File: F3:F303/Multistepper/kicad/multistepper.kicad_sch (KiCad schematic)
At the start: 14 parts, among them J8 USB_B, J9 Screw_Terminal_01x03, Q1 B0505S, SW3 SW_DIP_x01, U2 ISO1050DUB, U3 USBLC6-2SC6

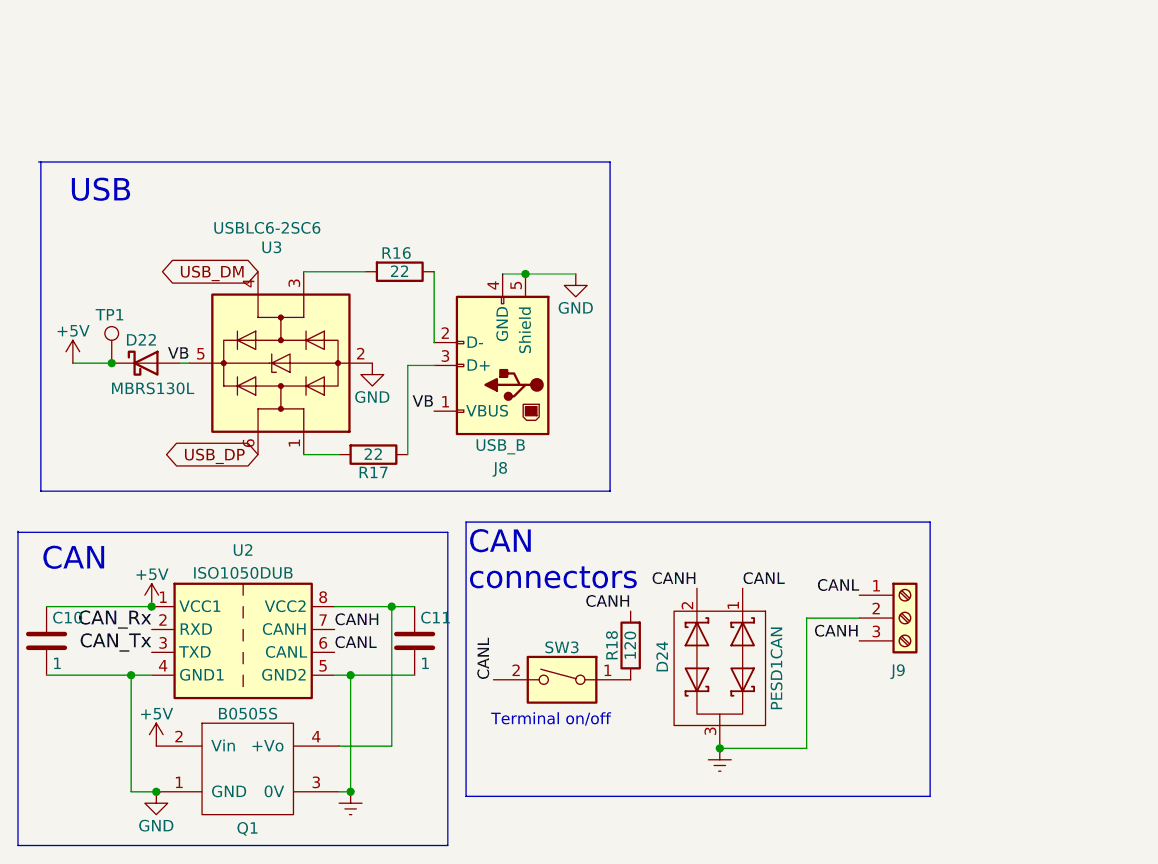
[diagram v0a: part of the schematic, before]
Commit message: multistepper: cont
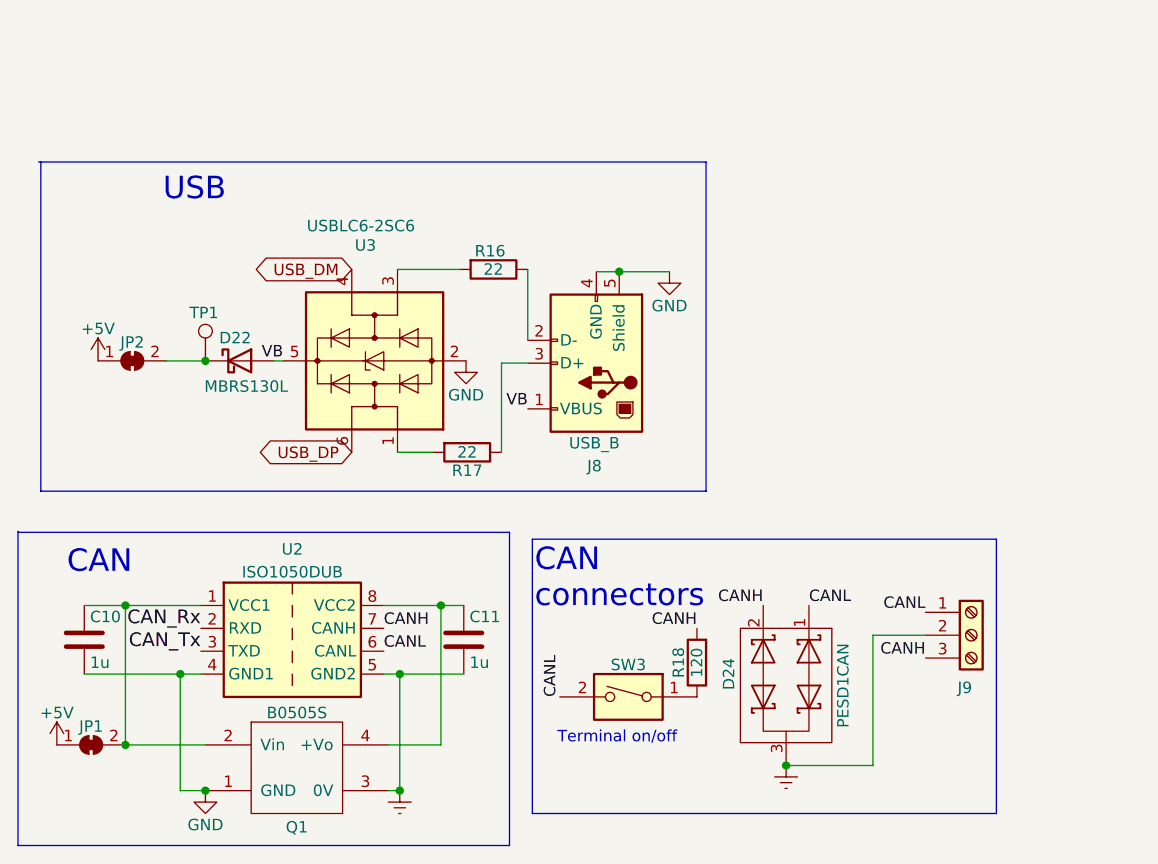
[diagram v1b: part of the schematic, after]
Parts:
- added JP1, JP2: SolderJumper_2_Bridged, Jumper:SolderJumper-2_P1.3mm_Open_TrianglePad1.0x1.5mm, symbol Jumper:SolderJumper_2_Bridged
- C10, C11: value 1 -> 1u; footprint Capacitor_SMD:C_0805_2012Metric_Pad1.15x1.40mm_HandSolder -> Capacitor_SMD:C_0603_1608Metric_Pad1.08x0.95mm_HandSolder
- Q1: footprint my_footprints:B0x0xS -> stepper:B0x0xS
- R16, R17: footprint Resistor_SMD:R_0603_1608Metric_Pad1.05x0.95mm_HandSolder -> Resistor_SMD:R_0603_1608Metric_Pad0.98x0.95mm_HandSolder
- R18: footprint Resistor_SMD:R_1210_3225Metric_Pad1.42x2.65mm_HandSolder -> Resistor_SMD:R_1210_3225Metric_Pad1.30x2.65mm_HandSolder
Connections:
- net +5V: now also JP1.1 (A), JP2.1 (A); no longer C10.1, D22.1 (K), Q1.2 (Vin), TP1.1, U2.1 (VCC1)
- new net: D22.1 (K), JP2.2 (B), TP1.1
- new net: C10.1, JP1.2 (B), Q1.2 (Vin), U2.1 (VCC1)
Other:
- moved on the sheet: C10, C11, D22, D24, J8, J9, Q1, R16, R17, R18, SW3, TP1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

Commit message: multistepper schematic
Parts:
- TP1: value 5V -> 5Vusb
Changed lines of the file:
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@@
       (effects (font (size 1.27 1.27)) (justify left))
     )
-    (property "Value" "5V" (id 1) (at 37.7952 139.7762 0)
+    (property "Value" "5Vusb" (id 1) (at 37.7952 139.7762 0)
       (effects (font (size 1.27 1.27)) (justify left) hide)
     )
@@
       (reference "#PWR03") (unit 1) (value "GND") (footprint "")
     )
-    (path "/076c38b6-e164-46bb-9d96-26f8bdfeca37/99206ade-04b2-46fa-85f1-261359dfd31b"
-      (reference "#PWR04") (unit 1) (value "+3V3") (footprint "")
-    )
     (path "/076c38b6-e164-46bb-9d96-26f8bdfeca37/f5301934-7edc-46db-ae48-58199dc2aa43"
       (reference "#PWR05") (unit 1) (value "GND") (footprint "")
@@
       (reference "#PWR08") (unit 1) (value "+3V3") (footprint "")
     )
-    (path "/076c38b6-e164-46bb-9d96-26f8bdfeca37/2b033d26-211f-47c5-ad30-9cb9aea659a6"
-      (reference "#PWR09") (unit 1) (value "+3V3") (footprint "")
-    )
-    (path "/076c38b6-e164-46bb-9d96-26f8bdfeca37/73b1df7f-a887-48b4-9ce7-3d8db7403e95"
-      (reference "#PWR010") (unit 1) (value "+3V3") (footprint "")
-    )
     (path "/076c38b6-e164-46bb-9d96-26f8bdfeca37/4d6a594b-d668-48f8-8d40-146959ef7aa5"
       (reference "#PWR011") (unit 1) (value "GND") (footprint "")
@@
       (reference "#PWR041") (unit 1) (value "GND") (footprint "")
     )
-    (path "/cf2c4fa9-a57e-4812-ae0c-3db57f6071a5/610893b8-7125-40df-867c-22854f8efd58/4f508297-4488-4315-85eb-5261f9d02134"
-      (reference "#PWR042") (unit 1) (value "+3.3V") (footprint "")
+    (path "/076c38b6-e164-46bb-9d96-26f8bdfeca37/4354a899-4f12-4b14-9a0f-0357b172479a"
+      (reference "#PWR042") (unit 1) (value "GND") (footprint "")
     )
     (path "/076c38b6-e164-46bb-9d96-26f8bdfeca37/c9d2b617-3560-41ef-a3a7-a6d08311dfc5"
@@
       (reference "#PWR0124") (unit 1) (value "GND") (footprint "")
     )
-    (path "/076c38b6-e164-46bb-9d96-26f8bdfeca37/b26d12d8-b821-4fbb-bcf0-02f1fc523839"
-      (reference "#PWR0125") (unit 1) (value "+3V3") (footprint "")
-    )
     (path "/076c38b6-e164-46bb-9d96-26f8bdfeca37/b728d2bc-216a-439f-be0d-9040aecbd583"
       (reference "C1") (unit 1) (value "12") (footprint "Capacitor_SMD:C_0603_1608Metric_Pad1.08x0.95mm_HandSolder")
@@
     )
     (path "/076c38b6-e164-46bb-9d96-26f8bdfeca37/9eb0e3e4-2412-4862-9254-ebfae0e788ab"
-      (reference "J2") (unit 1) (value "buttons_I2C") (footprint "Connector_IDC:IDC-Header_2x05_P2.54mm_Vertical")
+      (reference "J2") (unit 1) (value "Buttons/I2C") (footprint "Connector_IDC:IDC-Header_2x05_P2.54mm_Vertical")
     )
     (path "/076c38b6-e164-46bb-9d96-26f8bdfeca37/3b30193d-b3cb-42a8-a75c-e3cbeadeeead"
-      (reference "J3") (unit 1) (value "screen") (footprint "Connector_IDC:IDC-Header_2x05_P2.54mm_Vertical")
+      (reference "J3") (unit 1) (value "Screen") (footprint "Connector_IDC:IDC-Header_2x05_P2.54mm_Vertical")
     )
     (path "/beac4271-940a-4bcd-9fa5-ece775a07d41/ad1d252e-a412-4fd5-af6f-3bf5db8aac83"
@@
     )
     (path "/076c38b6-e164-46bb-9d96-26f8bdfeca37/23242767-ce55-4623-97c5-9de9c42c2a3f"
-      (reference "J7") (unit 1) (value "ADC2") (footprint "Connector_JST:JST_PH_B4B-PH-K_1x04_P2.00mm_Vertical")
+      (reference "J7") (unit 1) (value "GPO") (footprint "Connector_JST:JST_PH_B4B-PH-K_1x04_P2.00mm_Vertical")
     )
     (path "/0fd87c97-8042-4653-abdd-7019b1430685"
@@
       (reference "J10") (unit 1) (value "Screw_Terminal_01x02") (footprint "TerminalBlock_Phoenix:TerminalBlock_Phoenix_MKDS-1,5-2_1x02_P5.00mm_Horizontal")
     )
-    (path "/cf2c4fa9-a57e-4812-ae0c-3db57f6071a5/610893b8-7125-40df-867c-22854f8efd58/0f165469-1249-4064-aadf-0fc6a85a60f4"
-      (reference "J11") (unit 1) (value "Conn_01x03_Male") (footprint "Connector_PinHeader_2.54mm:PinHeader_1x03_P2.54mm_Vertical")
-    )
     (path "/cf2c4fa9-a57e-4812-ae0c-3db57f6071a5/610893b8-7125-40df-867c-22854f8efd58/0f3f2180-6e00-4de5-8d6d-bb200c241b76"
-      (reference "J12") (unit 1) (value "Conn_01x03_Male") (footprint "Connector_PinHeader_2.54mm:PinHeader_1x03_P2.54mm_Vertical")
+      (reference "J11") (unit 1) (value "LimS") (footprint "Connector_JST:JST_EH_B4B-EH-A_1x04_P2.50mm_Vertical")
     )
     (path "/cf2c4fa9-a57e-4812-ae0c-3db57f6071a5/610893b8-7125-40df-867c-22854f8efd58/e602956b-fb1a-48e1-af9c-9935214ce0ab"
-      (reference "J13") (unit 1) (value "Conn_01x04_Male") (footprint "Connector_PinHeader_2.54mm:PinHeader_1x04_P2.54mm_Vertical")
+      (reference "J12") (unit 1) (value "Stepper") (footprint "Connector_JST:JST_EH_B4B-EH-A_1x04_P2.50mm_Vertical")
+    )
+    (path "/076c38b6-e164-46bb-9d96-26f8bdfeca37/8a056ff3-5fc5-445e-813f-5479481ae2be"
+      (reference "J13") (unit 1) (value "UART") (footprint "Connector_JST:JST_PH_B3B-PH-K_1x03_P2.00mm_Vertical")
     )
     (path "/e07df136-9c14-457d-8c74-2e7051ea67ac"
@@
       (reference "JP15") (unit 1) (value "SolderJumper_2_Bridged") (footprint "Jumper:SolderJumper-2_P1.3mm_Open_TrianglePad1.0x1.5mm")
     )
-    (path "/cf2c4fa9-a57e-4812-ae0c-3db57f6071a5/610893b8-7125-40df-867c-22854f8efd58/19b709bd-064d-431e-981a-21d8140226f7"
-      (reference "JP16") (unit 1) (value "SolderJumper_2_Bridged") (footprint "Jumper:SolderJumper-2_P1.3mm_Open_TrianglePad1.0x1.5mm")
-    )
-    (path "/cf2c4fa9-a57e-4812-ae0c-3db57f6071a5/610893b8-7125-40df-867c-22854f8efd58/9a737b0c-0674-4408-94a4-2d0cb4f1ebe2"
-      (reference "JP17") (unit 1) (value "SolderJumper_2_Bridged") (footprint "Jumper:SolderJumper-2_P1.3mm_Open_TrianglePad1.0x1.5mm")
-    )
     (path "/916f71ef-9b2f-424f-a64d-0b6af99b627f/b3fc53d8-12ed-4d5b-adca-e33d10eb8430"
       (reference "L1") (unit 1) (value "100u") (footprint "Inductor_THT:L_Toroid_Horizontal_D6.5mm_P10.00mm_Diameter7-5mm_Amidon-T25")
@@
       (reference "R23") (unit 1) (value "100") (footprint "Resistor_SMD:R_0603_1608Metric_Pad0.98x0.95mm_HandSolder")
     )
+    (path "/076c38b6-e164-46bb-9d96-26f8bdfeca37/d42c91a2-1307-4ab7-930f-7f9359c5d693"
+      (reference "R24") (unit 1) (value "22") (footprint "Resistor_SMD:R_0603_1608Metric_Pad0.98x0.95mm_HandSolder")
+    )
+    (path "/076c38b6-e164-46bb-9d96-26f8bdfeca37/a8f0ad58-076a-43bc-8bc2-4c8514b9f66a"
+      (reference "R25") (unit 1) (value "22") (footprint "Resistor_SMD:R_0603_1608Metric_Pad0.98x0.95mm_HandSolder")
+    )
     (path "/076c38b6-e164-46bb-9d96-26f8bdfeca37/c2620a21-1c3d-4233-bbce-d374c7c78b67"
       (reference "RN1") (unit 1) (value "330") (footprint "Resistor_SMD:R_Array_Convex_4x0603")
@@
     )
     (path "/076c38b6-e164-46bb-9d96-26f8bdfeca37/28ab1d00-5dcf-4df3-bb52-f6a6fa59c5a0"
-      (reference "SW1") (unit 1) (value "reset") (footprint "Button_Switch_SMD:SW_SPST_FSMSM")
+      (reference "SW1") (unit 1) (value "Reset") (footprint "Button_Switch_SMD:SW_SPST_FSMSM")
     )
     (path "/076c38b6-e164-46bb-9d96-26f8bdfeca37/7c777c8b-6b38-45e7-b24d-d876b91caf36"
-      (reference "SW2") (unit 1) (value "boot") (footprint "Button_Switch_SMD:SW_SPST_FSMSM")
+      (reference "SW2") (unit 1) (value "Boot") (footprint "Button_Switch_SMD:SW_SPST_FSMSM")
     )
     (path "/b27ea6a0-a572-46ba-ba2a-053475cc4a03"
@@
     )
     (path "/fa927120-76d0-4789-86fa-35db42ec6d7f"
-      (reference "TP1") (unit 1) (value "5V") (footprint "TestPoint:TestPoint_THTPad_1.5x1.5mm_Drill0.7mm")
+      (reference "TP1") (unit 1) (value "5Vusb") (footprint "TestPoint:TestPoint_THTPad_1.5x1.5mm_Drill0.7mm")
     )
     (path "/916f71ef-9b2f-424f-a64d-0b6af99b627f/84be84b6-c711-4dd0-ad57-498504d82650"
